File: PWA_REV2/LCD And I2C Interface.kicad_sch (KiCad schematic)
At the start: 44 parts, among them Q301 BSS138, Q401 BSS138, Q402 BSS138, U301 PCF8574AT_3_518, U302 LCD_20x4_Character-GPAD_SCH_L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, U303 Conn_01x16

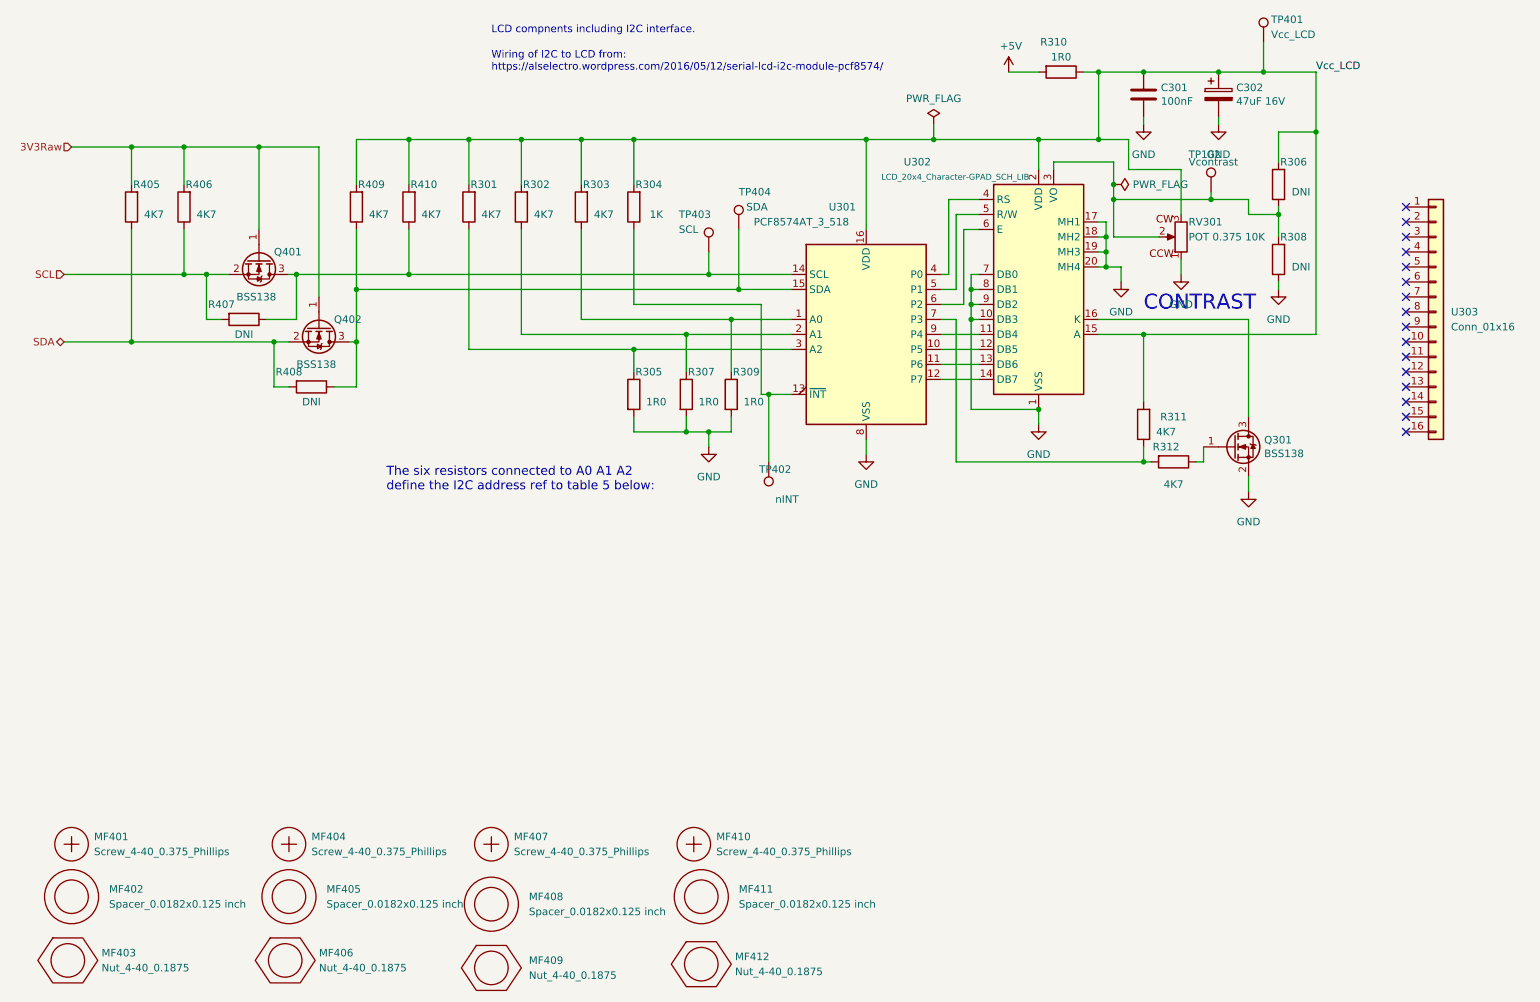
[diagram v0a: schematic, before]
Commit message: PWA_REV2.kicad, clearing ERC warning by replacing the spacer and the potentiometer with its identicle from the GPAD_SCH_LIB library.
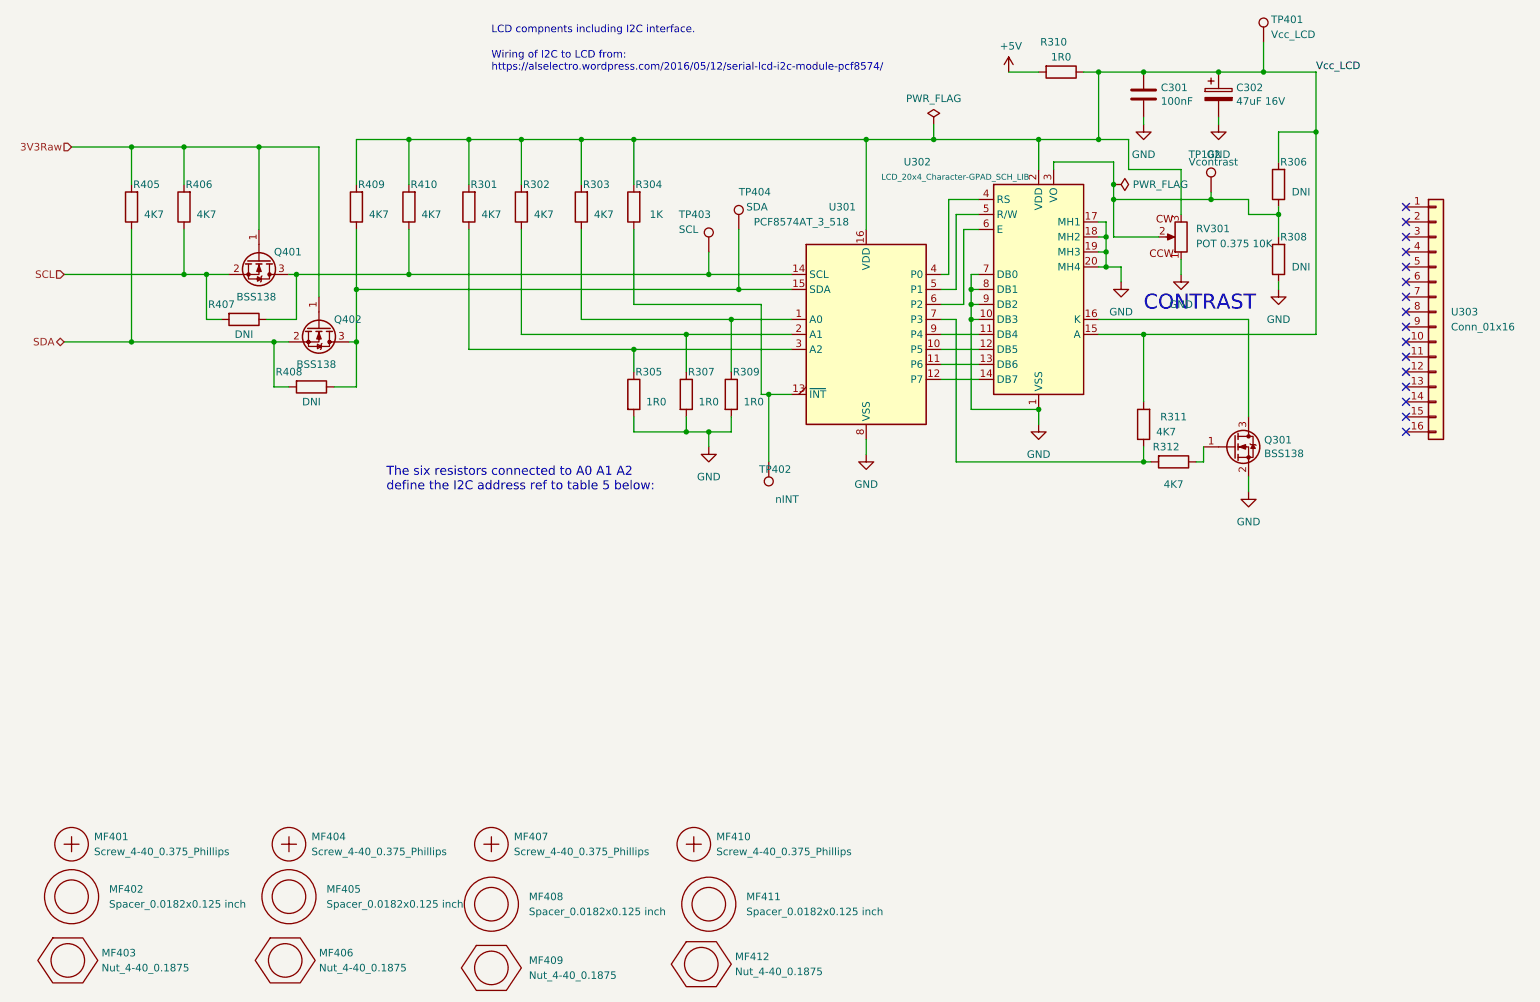
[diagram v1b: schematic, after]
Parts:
- removed MF402, MF405, MF408, MF411: Spacer_0.0182x0.125 inch, symbol GPAD_SCH_LIB:Spacer_0.0182x0.125 inch
- removed RV301: POT 0.375 10K, GeneralPurposeAlarmDevicePCB:Potentiometer_Bourns_3386P_Vertical, symbol GPAD_SCH_LIB:POT 0.375 10K
- added MF402, MF405, MF408, MF411: Spacer_0.0182x0.125 inch, symbol GPAD_SCH_LIB:Spacer_0.0182x0.125_inch
- added RV301: POT 0.375 10K, GeneralPurposeAlarmDevicePCB:Potentiometer_Bourns_3386P_Vertical, symbol GPAD_SCH_LIB:POT_0.375_10K
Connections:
- net GND: now also RV301.1
- net Vcc_LCD: now also RV301.3
- net at R306.1, R308.2, TP102.1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: now also RV301.2
